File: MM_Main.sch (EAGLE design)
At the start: 82 parts, among them IC1 ULN2003AD, IC2 TB6612FNG, IC4 LD117ADT50TR, IC5 MCP1825, Q1 TEFT4300, Q2 TEFT4300, Q3 TEFT4300, Q4 TEFT4300, Q5 TEFT4300, Q6 TEFT4300, Q7 8MHz

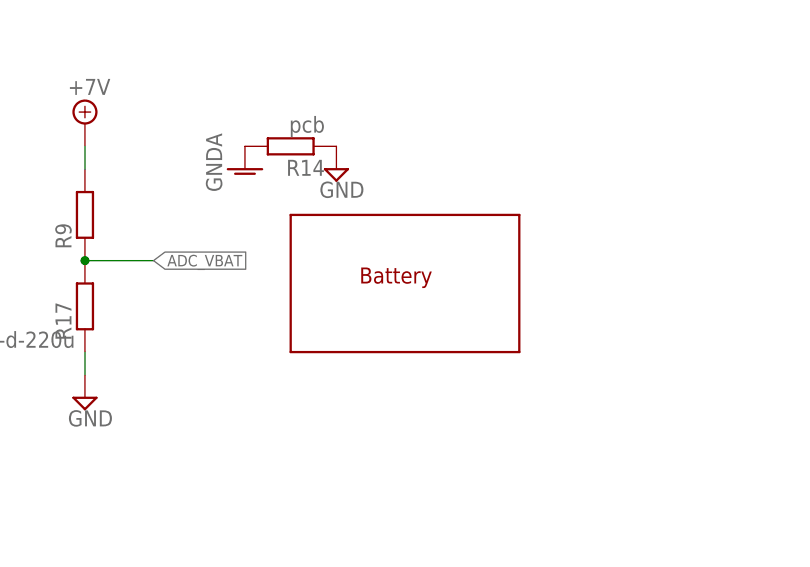
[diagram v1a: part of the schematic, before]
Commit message: poprawki warst opisowych, dodanie gerberow mm
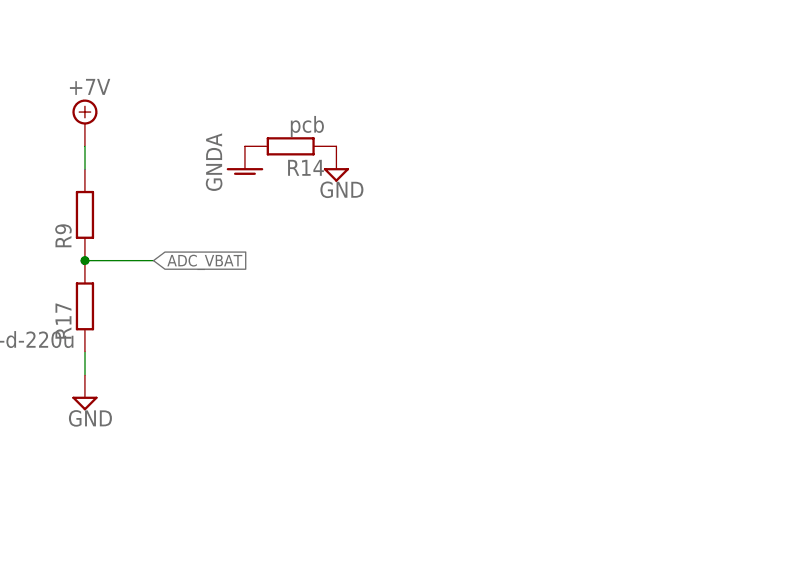
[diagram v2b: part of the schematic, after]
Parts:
- removed U$2: LI-POL-DUALKSY_220MAH_D, _microMouse:LI-POL-DUALKSY_220MAH_D
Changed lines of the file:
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@@
 <part name="ZAS" library="special" deviceset="SW_DIP-1" device=""/>
 <part name="FUSE" library="resistor" deviceset="R-EU_" device="M2012"/>
-<part name="U$2" library="_microMouse" deviceset="LI-POL" device="-DUALKSY_220MAH_D" value="LI-POL-DUALKSY_220MAH_D"/>
 <part name="U$1" library="_microMouse" deviceset="9AXIS_MODULE" device=""/>
 <part name="+3V1" library="supply1" deviceset="+3V3" device=""/>
@@
 <instance part="ZAS" gate="G$1" x="-139.7" y="121.92" rot="R180"/>
 <instance part="FUSE" gate="G$1" x="-127" y="121.92" rot="R180"/>
-<instance part="U$2" gate="G$1" x="-71.12" y="121.92"/>
 <instance part="U$1" gate="G$1" x="358.14" y="76.2"/>
 <instance part="+3V1" gate="G$1" x="-12.7" y="40.64"/>
